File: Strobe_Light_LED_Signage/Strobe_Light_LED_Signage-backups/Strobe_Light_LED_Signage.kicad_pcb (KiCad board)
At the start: 2 copper layers, 100 x 80 mm, 137 parts, among them J1 Conn_01x04_Socket, J2 USB_B_Micro, J3 Conn_01x02_Socket, J4 Conn_01x02_Socket, J5 Conn_01x02_Socket, J6 Screw_Terminal_01x16, J7 Screw_Terminal_01x16, J8 Conn_01x02_Socket, J9 Conn_01x03_Socket, K1 EE2-5NU, K2 EE2-5NU, K3 EE2-5NU, K4 EE2-5NU, K5 EE2-5NU, K7 EE2-5NU, Q1 BSS138, Q2 BSS138, Q3 Q_NPN_BEC, Q4 Q_NPN_BEC, Q5 Q_NPN_BEC, Q6 Q_NPN_BEC, Q7 Q_NPN_BEC, Q9 Q_NPN_BEC, SW1 SW_Push, SW2 SW_Push, U1 LM2596S-5, U2 CH340C, U3 ESP32-WROOM-32, U4 74HC595, U5 AMS1117-3.3, U6 MAX485E, U7 TPL5010

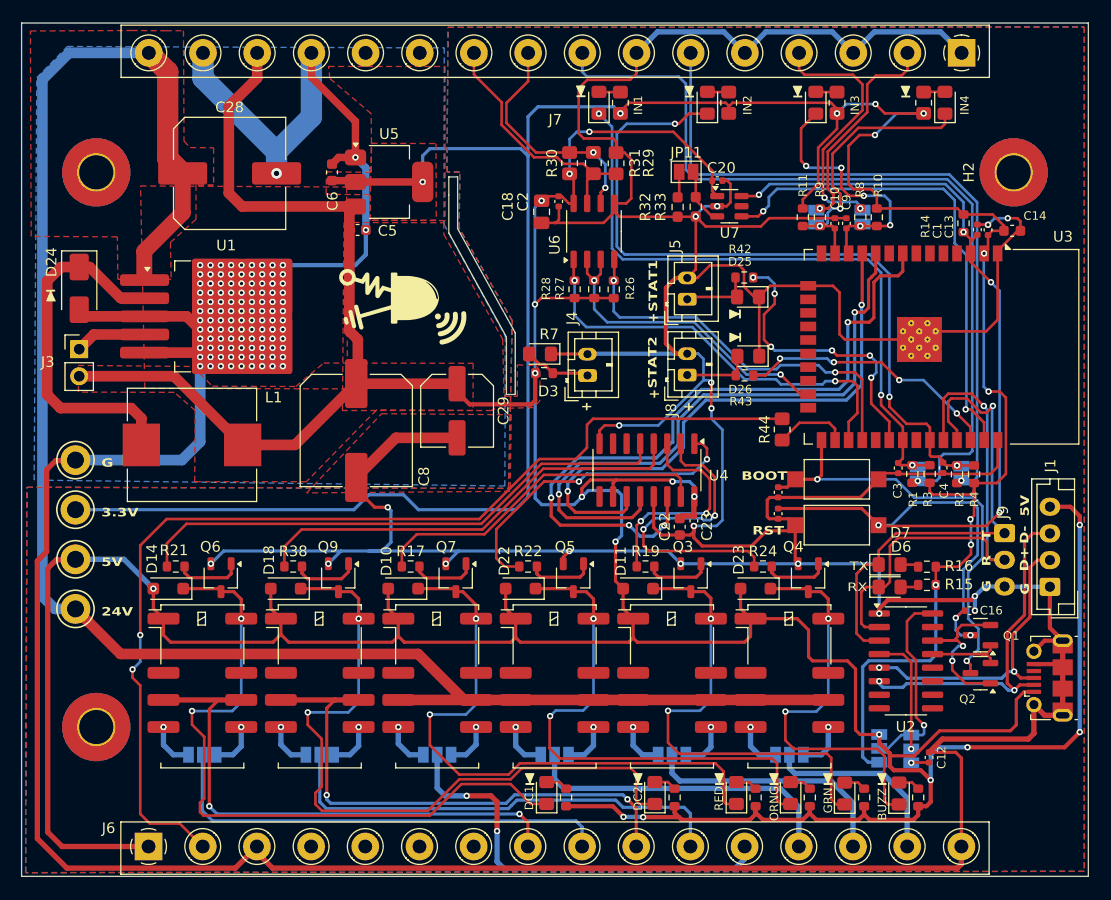
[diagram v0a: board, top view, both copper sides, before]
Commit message: Version 1.0 of both Strobe Light and PLC Done
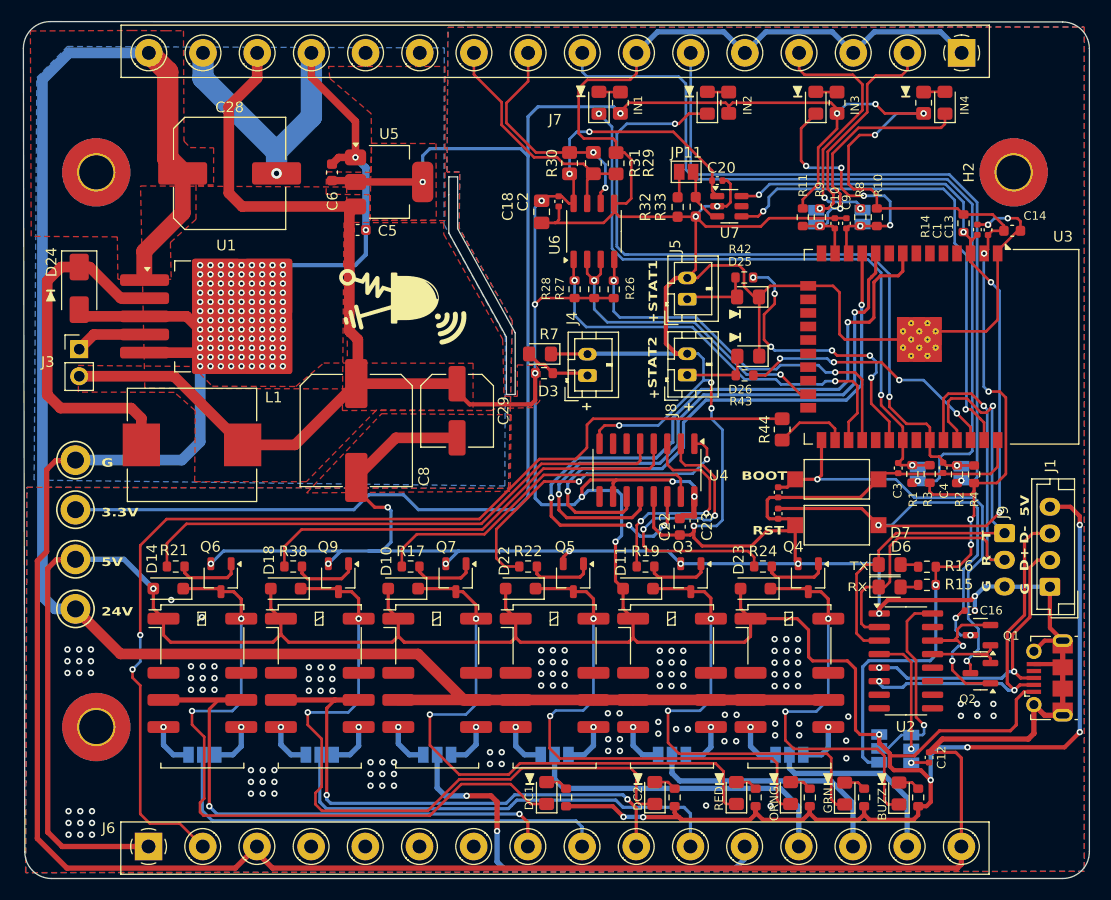
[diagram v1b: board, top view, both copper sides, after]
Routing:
- net GND: vias 129 -> 257
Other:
- board size 100 x 80 mm -> 99.9 x 80.3 mm
